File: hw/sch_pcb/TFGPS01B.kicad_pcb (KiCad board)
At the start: 4 copper layers, 51 x 51 mm, 74 parts, among them J1 SM10B-GHS-TB, J2 USBC_USB4105-GF-A, J3 SM06B-GHS-TB, J4 SM04B-GHS-TB, J5 SM08B-GHS-TB, M1 HOLE, M2 HOLE, M3 HOLE, M4 HOLE, Q1 BC817-25, Q2 BC817-25, Q3 BC817-25, U1 MIC5504-3.3YM5, U2 USBLC6-2SC6, U3 NEO-M8P, U4 MAX2655

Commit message: Edit PCB
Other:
- rule pad_to_mask_clearance: 0 -> 0.2
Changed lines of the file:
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@@
       (dielectric_constraints no)
     )
-    (pad_to_mask_clearance 0)
+    (pad_to_mask_clearance 0.2)
     (pcbplotparams
       (layerselection 0x00010e0_ffffffff)

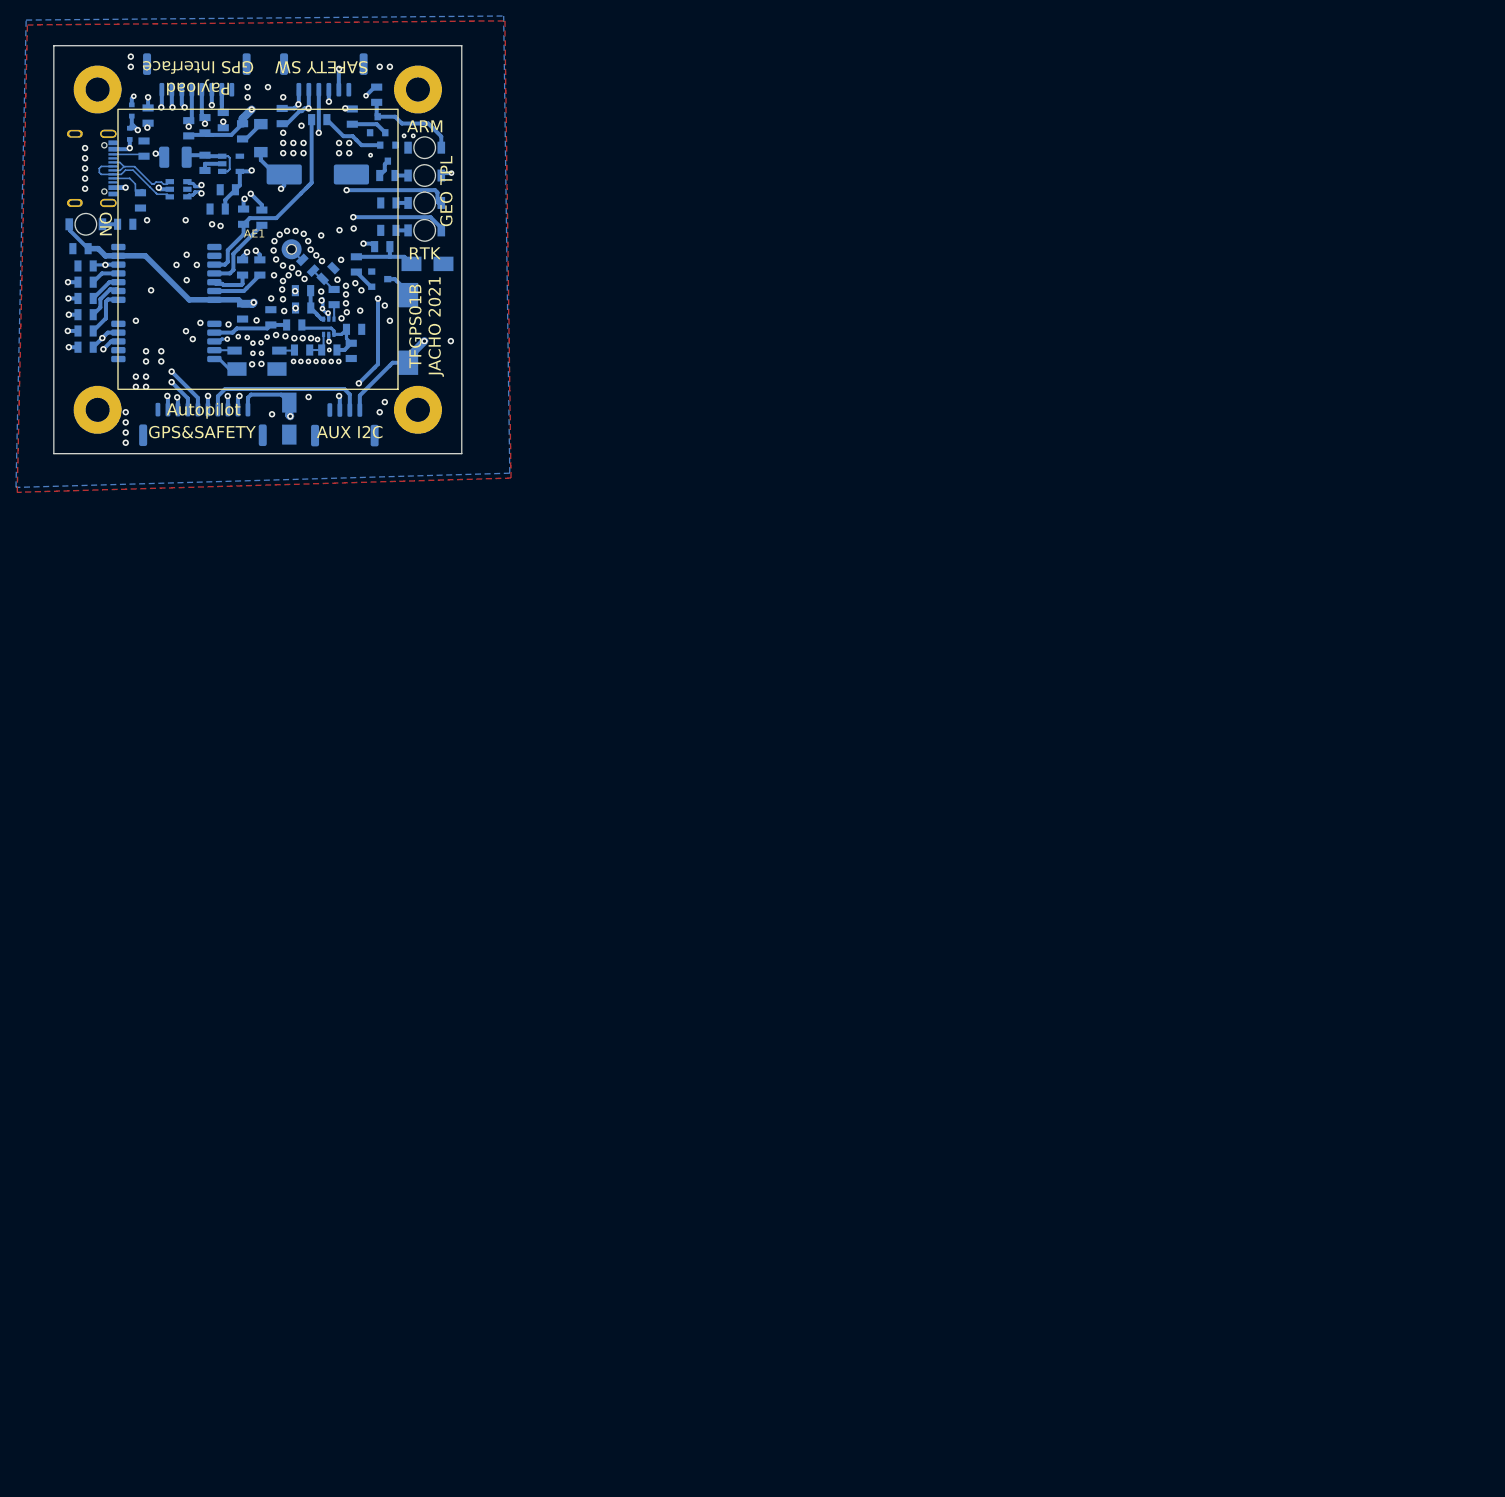
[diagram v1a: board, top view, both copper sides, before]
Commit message: Uprava projektovych dat
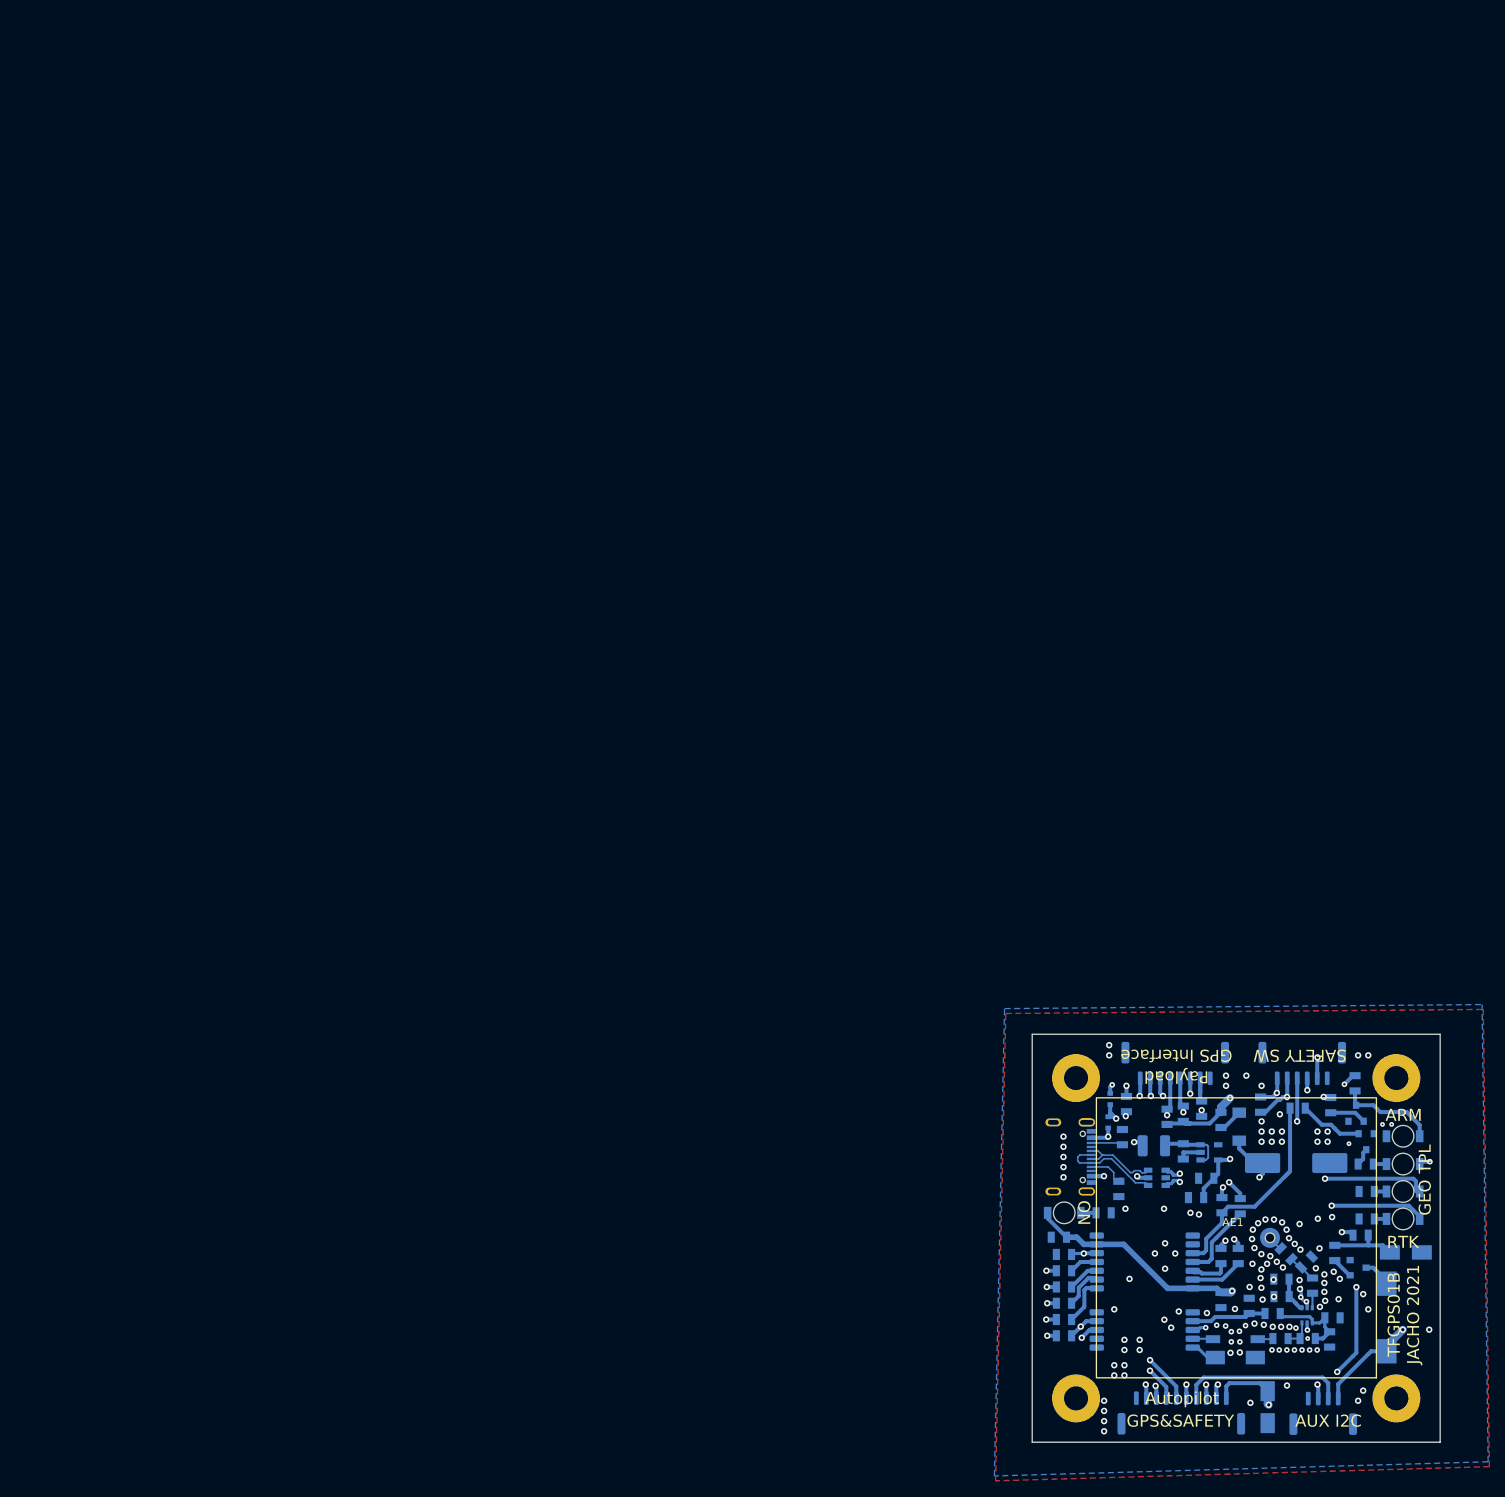
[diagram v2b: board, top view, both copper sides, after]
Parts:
- moved C13 173.9 mm to (156.5, 101.1)
- moved C3 173.9 mm to (141.1, 87.3)
- moved C9 173.9 mm to (159.7, 108.1)
- moved D4 173.9 mm to (168.6, 88.9)
- moved D5 173.9 mm to (168.6, 92.3)
- moved D6 173.9 mm to (168.6, 95.8)
- moved D7 173.9 mm to (168.6, 85.4)
- moved D9 173.9 mm to (132.0, 80.8)
- moved FL1 173.9 mm to (147.6, 110.8)
- moved L1 173.9 mm to (137.4, 86.6)
- moved L2 173.9 mm to (157.2, 104.1)
- moved M2 173.9 mm to (127.7, 118.2)
- moved M4 173.9 mm to (167.7, 118.2)
- moved Q3 173.9 mm to (162.7, 82.5)
- moved R13 173.9 mm to (155.4, 81.9)
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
